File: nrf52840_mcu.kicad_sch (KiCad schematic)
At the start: 36 parts, among them U5 ZD25WQ16CTIGT, U6 NRF52840-QIAA-R, X1 S201632M10PF10PPM, Y1 32.768KHz

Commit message: WIP: Moved buttons, battery.
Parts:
- L1: Resource (none) -> https://muehlhaus.com/support/antenna/ceramic-antenna
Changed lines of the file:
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@@
+			)
+		)
+		(property "Resource" "https://muehlhaus.com/support/antenna/ceramic-antenna"
+			(at 27.94 173.99 0)
+			(effects
+				(font
+					(size 1.27 1.27)
+				)
+				(hide yes)
 			)
 		)

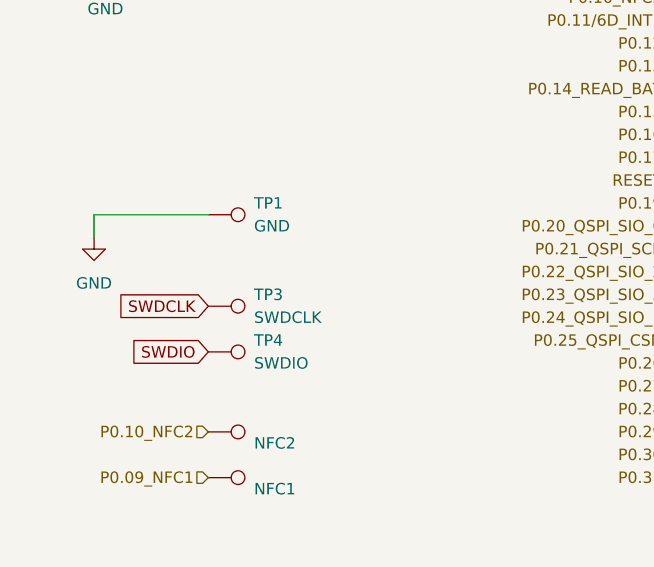
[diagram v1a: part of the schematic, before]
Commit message: Add JTAG 2.54mm header footprint.
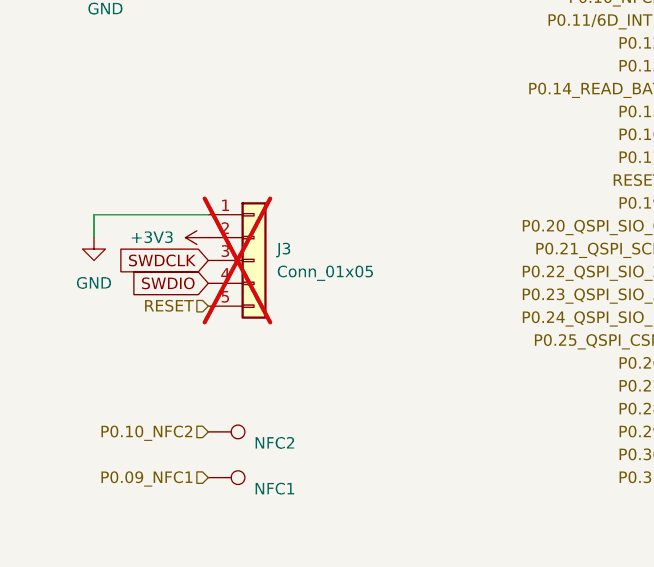
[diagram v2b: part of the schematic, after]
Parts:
- removed TP1: GND, TestPoint:TestPoint_Pad_D1.5mm, symbol Connector:TestPoint
- removed TP3: SWDCLK, TestPoint:TestPoint_Pad_D1.5mm, symbol Connector:TestPoint
- removed TP4: SWDIO, TestPoint:TestPoint_Pad_D1.5mm, symbol Connector:TestPoint
- added J3: Conn_01x05, Connector_PinHeader_2.54mm:PinHeader_1x05_P2.54mm_Vertical, symbol Connector_Generic:Conn_01x05
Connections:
- net +3V3: now also J3.2 (Pin_2)
- net GND: now also J3.1 (Pin_1)
- net RESET: now also J3.5 (Pin_5)
- net SWDCLK: now also J3.3 (Pin_3)
- net SWDIO: now also J3.4 (Pin_4)

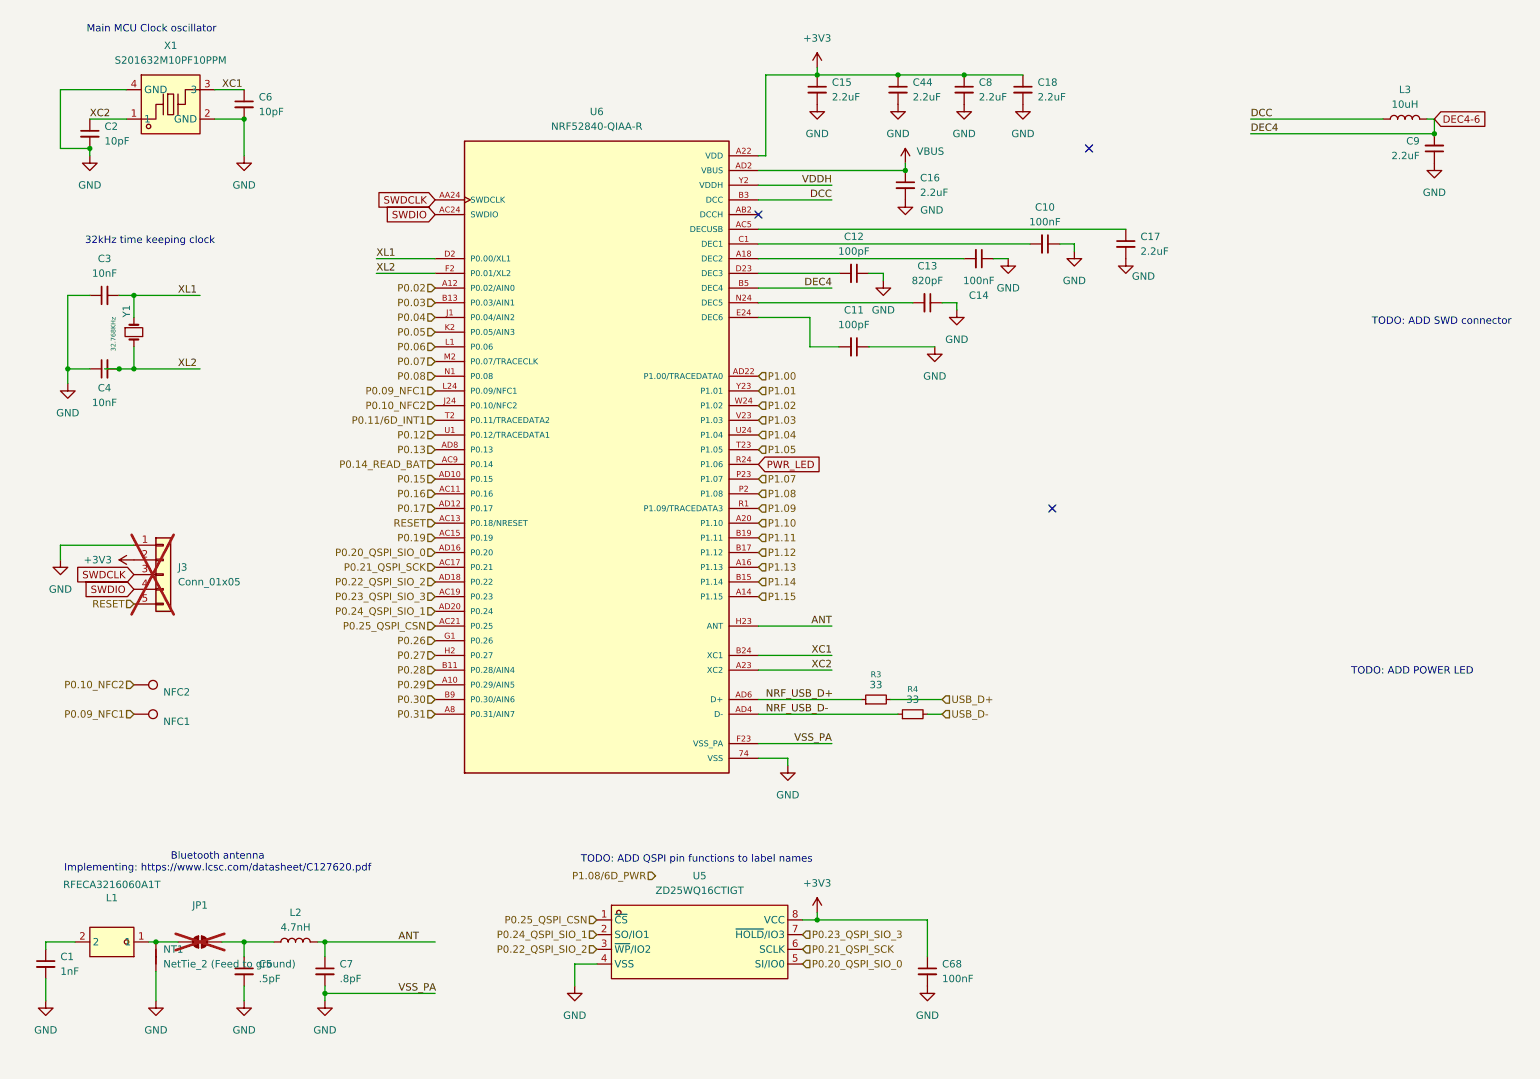
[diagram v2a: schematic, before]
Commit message: Check & fix MCU schematic
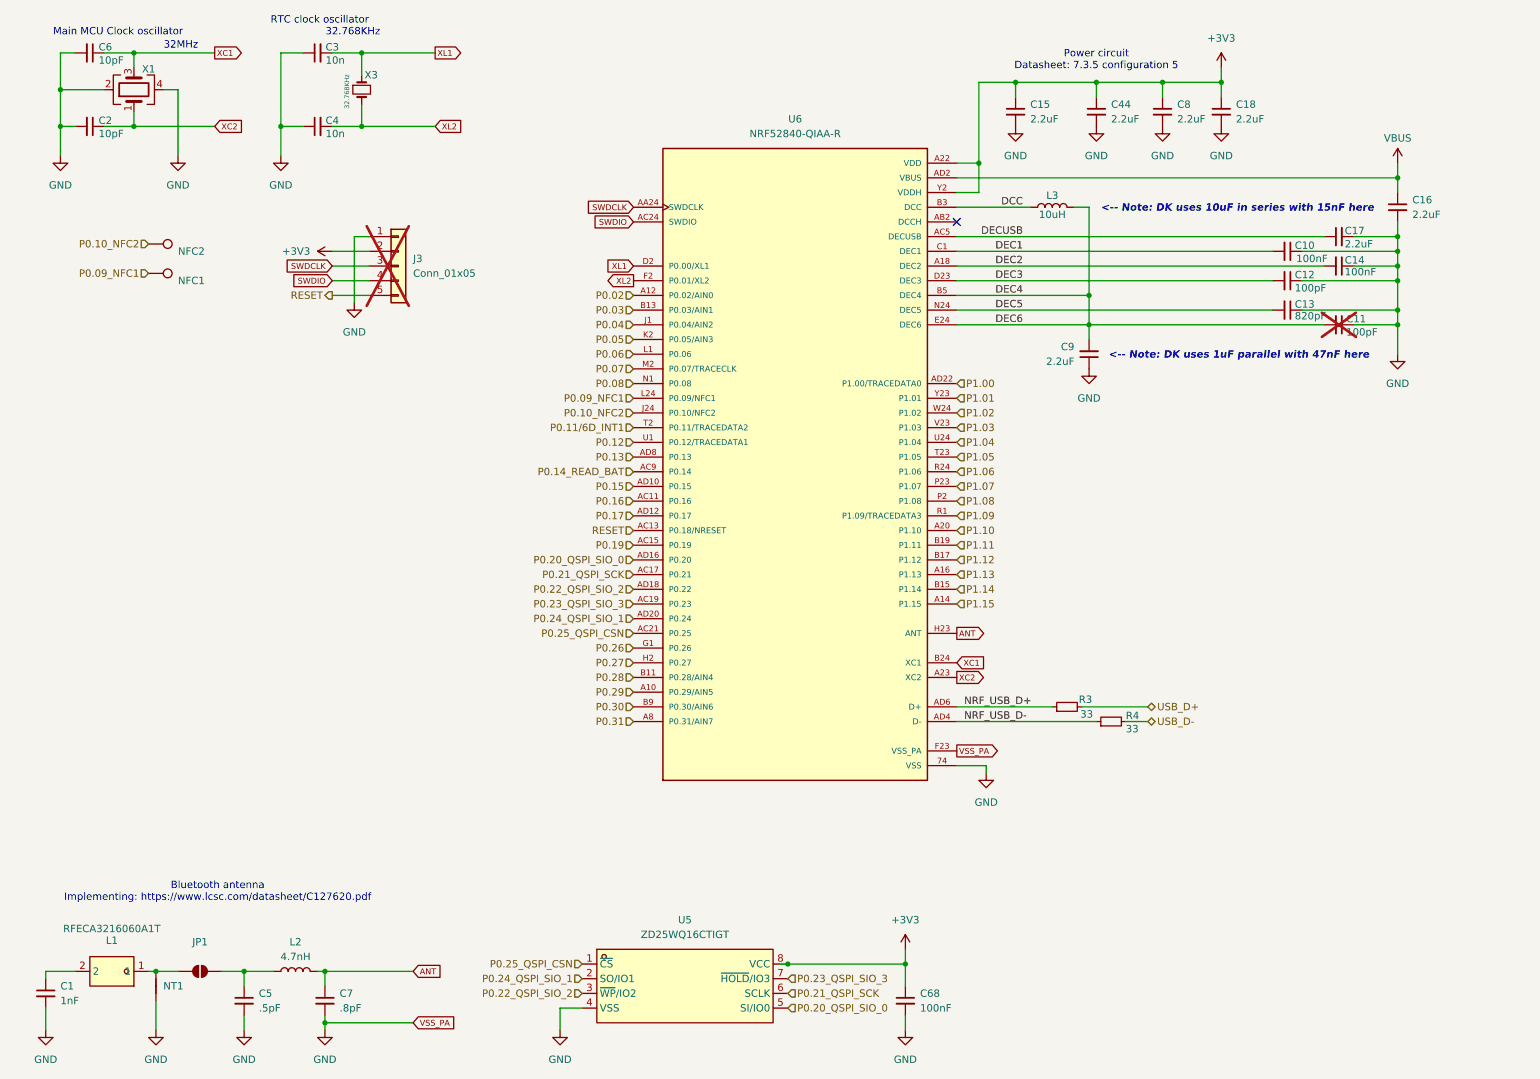
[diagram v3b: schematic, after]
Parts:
- C11: now not fitted; now left out of the parts list
- C3, C4: value 10nF -> 10n
- JP1: now fitted
- X1: symbol lcsc:S201632M10PF10PPM -> Device:Crystal_GND24
- renumbered Y1 to X3
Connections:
- net DEC4-6 is gone; now on net DEC4: C9.2, L3.1, U6.B5 (DEC4)
- net VDDH is gone; now on net +3V3: U6.Y2 (VDDH)
- net DEC3: now reaches C12.2, U6.D23 (DEC3)
- net DEC4: now reaches C11.2, U6.E24 (DEC6)
- net DEC2: now reaches C14.2, U6.A18 (DEC2)
- net DECUSB: now reaches C17.1, U6.AC5 (DECUSB)
- net DEC1: now reaches C10.2, U6.C1 (DEC1)
- net DEC5: now reaches C13.2, U6.N24 (DEC5)
- net PWR_LED renamed P1.06
- no-connect marks 3 -> 1
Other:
- note added: "32.768KHz"
- note added: "32MHz"
- note added: "<-- Note: DK uses 10uF in series with 15nF here"
- note added: "<-- Note: DK uses 1uF parallel with 47nF here"
- note added: "Power circuit Datasheet: 7.3.5 configuration 5"
- note added: "RTC clock oscillator"
- note removed: "32kHz time keeping clock"
- note removed: "TODO: ADD POWER LED"
- note removed: "TODO: ADD QSPI pin functions to label names"
- note removed: "TODO: ADD SWD connector"
- moved on the sheet: C1, C10, C12, C13, C14, C15, C16, C17, C18, C2, C3, C4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

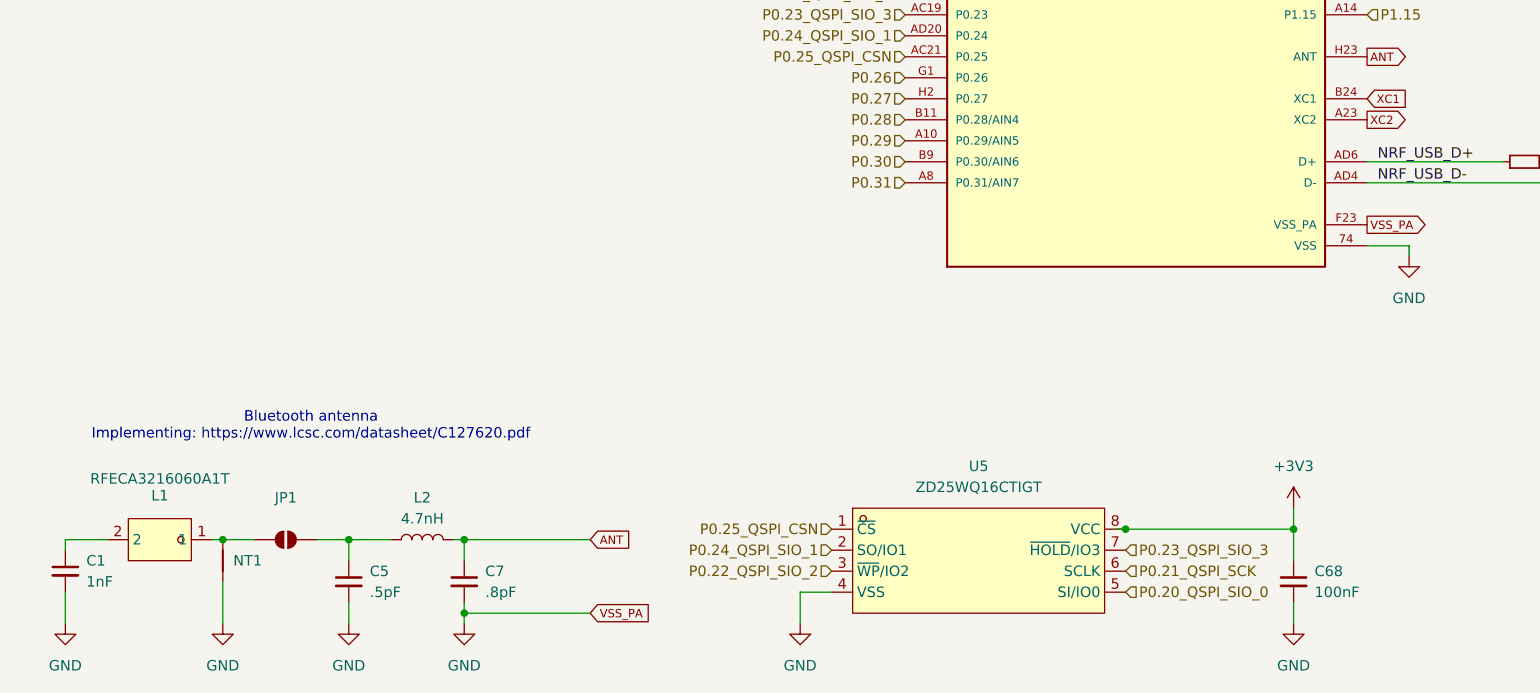
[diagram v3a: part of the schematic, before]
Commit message: Processed the unconnected pads in the NRF52 Renze found, Added the IPEX connector to allow tuning of the Bluetooth antenna, moved the RESET button.
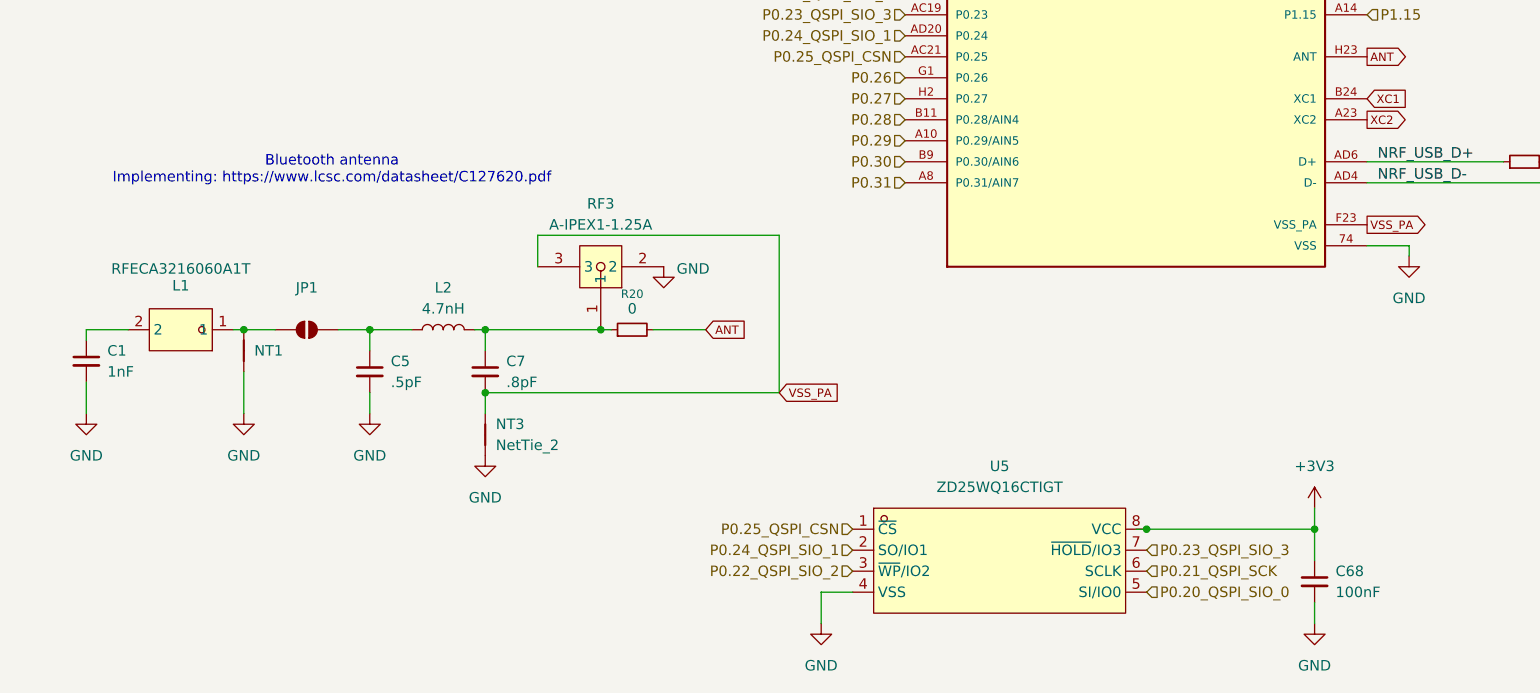
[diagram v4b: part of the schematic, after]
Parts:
- added NT3: NetTie_2, NetTie:NetTie-2_SMD_Pad0.5mm, symbol Device:NetTie_2
- added R20: 0, Resistor_SMD:R_0402_1005Metric, symbol Device:R_Small
- added RF3: A-IPEX1-1.25A, lcsc:IPEX-SMD_3P-L2.6-W2.6-LS3.0_RF1200001R, symbol lcsc:A-IPEX1-1.25A
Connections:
- net ANT: now also R20.2; no longer C7.1, L2.2
- net GND: now also NT3.1, RF3.2; no longer C7.2, U6.F23 (VSS_PA)
- new net: C7.1, L2.2, R20.1, RF3.1
- new net VSS_PA: C7.2, NT3.2, RF3.3, U6.F23 (VSS_PA)
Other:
- moved on the sheet: C1, C5, C68, C7, JP1, L1, L2, NT1, U5

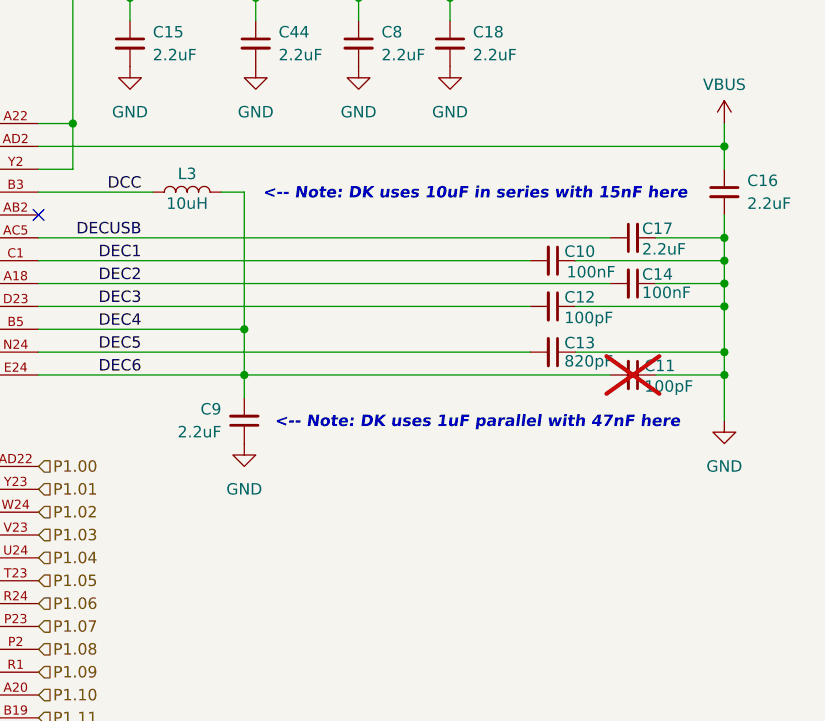
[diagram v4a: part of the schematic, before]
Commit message: Moved battery connector out of the way of the battery.
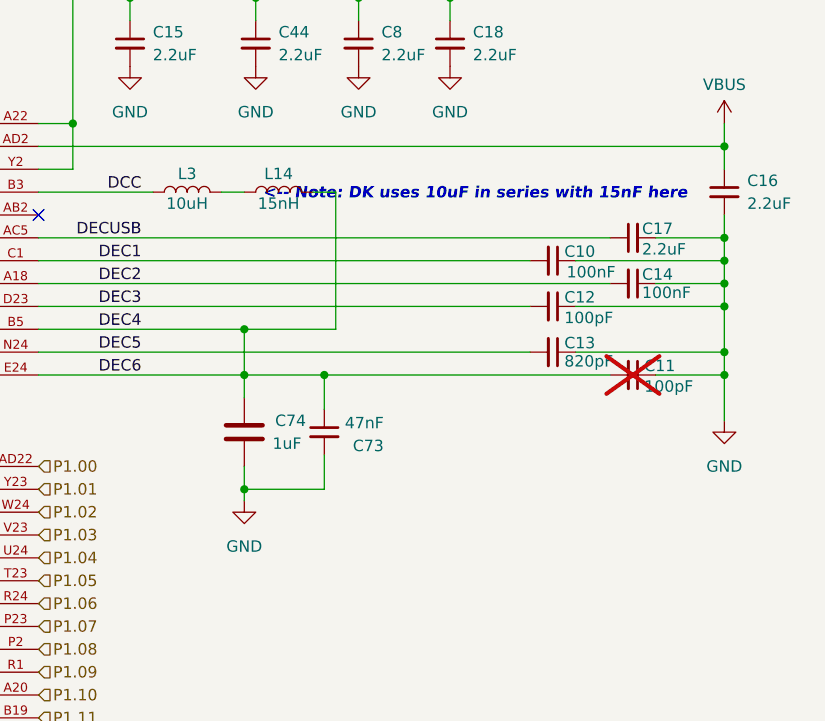
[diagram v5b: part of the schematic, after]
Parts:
- removed C9: 2.2uF, Capacitor_SMD:C_0402_1005Metric, symbol Device:C_Small
- added C73: 47nF, Capacitor_SMD:C_0402_1005Metric, symbol Device:C_Small
- added C74: 1uF, Capacitor_SMD:C_0603_1608Metric, symbol symbols:C
- added L14: 15nH, Inductor_SMD:L_0402_1005Metric, symbol Device:L
- L3: footprint Inductor_SMD:L_0805_2012Metric -> Inductor_SMD:L_0603_1608Metric; LCSC C95978 -> C194437
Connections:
- net DEC4: now also C73.1, C74.2, L14.1; no longer L3.1
- net GND: now also C73.2, C74.1
- new net: L14.2, L3.1
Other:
- note removed: "<-- Note: DK uses 1uF parallel with 47nF here"

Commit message: Checked PCBA for JLCPCB.
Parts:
- L1: LCSC (none) -> C127620
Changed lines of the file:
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@@
 			)
 		)
-		(property "Datasheet" "~"
+		(property "Datasheet" "https://jlcpcb.com/partdetail/SST-S201632M10PF10PPM/C7420782"
 			(at 31.75 26.67 0)
 			(effects
@@
 			)
 		)
+		(property "LCSC" "C127620"
+			(at 30.48 153.67 0)
+			(effects
+				(font
+					(size 1.27 1.27)
+				)
+				(hide yes)
+			)
+		)
 		(pin "2"
 		)
@@
 			)
 		)
-		(property "Datasheet" "https://www.lcsc.com/datasheet/C127620.pdf"
+		(property "Datasheet" "~"
 			(at 38.1 156.21 0)
 			(effects

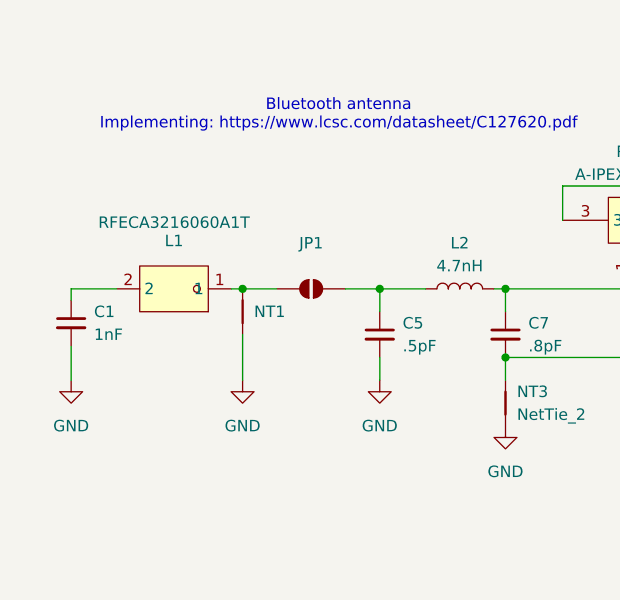
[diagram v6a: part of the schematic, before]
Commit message: Changed antennas for PCB antennas, move stuff because of it.
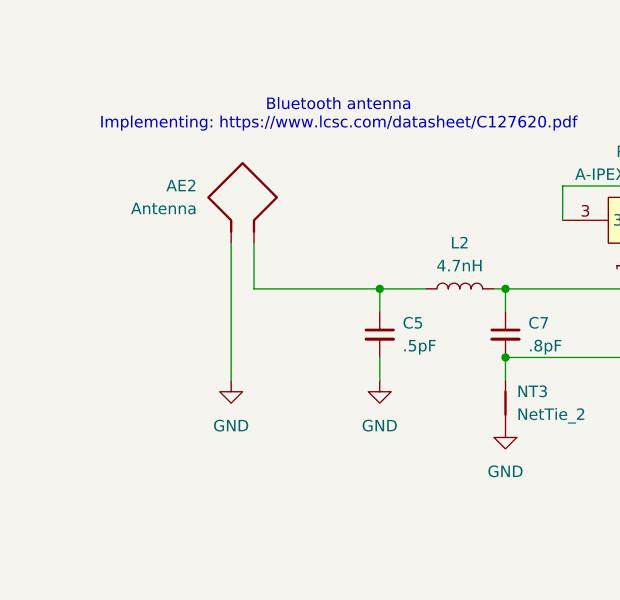
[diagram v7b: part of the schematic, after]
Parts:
- removed C1: 1nF, Capacitor_SMD:C_0402_1005Metric, symbol Device:C_Small
- removed JP1: SolderJumper_2_Open, symbol Jumper:SolderJumper_2_Open
- removed L1: RFECA3216060A1T, lcsc:ANT-SMD_L3.1-W1.6, symbol lcsc:RFECA3216060A1T
- removed NT1: NetTie_2 (Feed to ground), lcsc:NetTie-2_SMD_SQ_Pad0.8mm, symbol Device:NetTie_2
- added AE2: Antenna, RF_Antenna:Texas_SWRA117D_2.4GHz_Left, symbol Device:Antenna_Loop
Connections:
- net GND: now also AE2.2
- net at C5.1, L2.1: now also AE2.1
